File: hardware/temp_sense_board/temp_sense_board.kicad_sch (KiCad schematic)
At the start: 3 parts

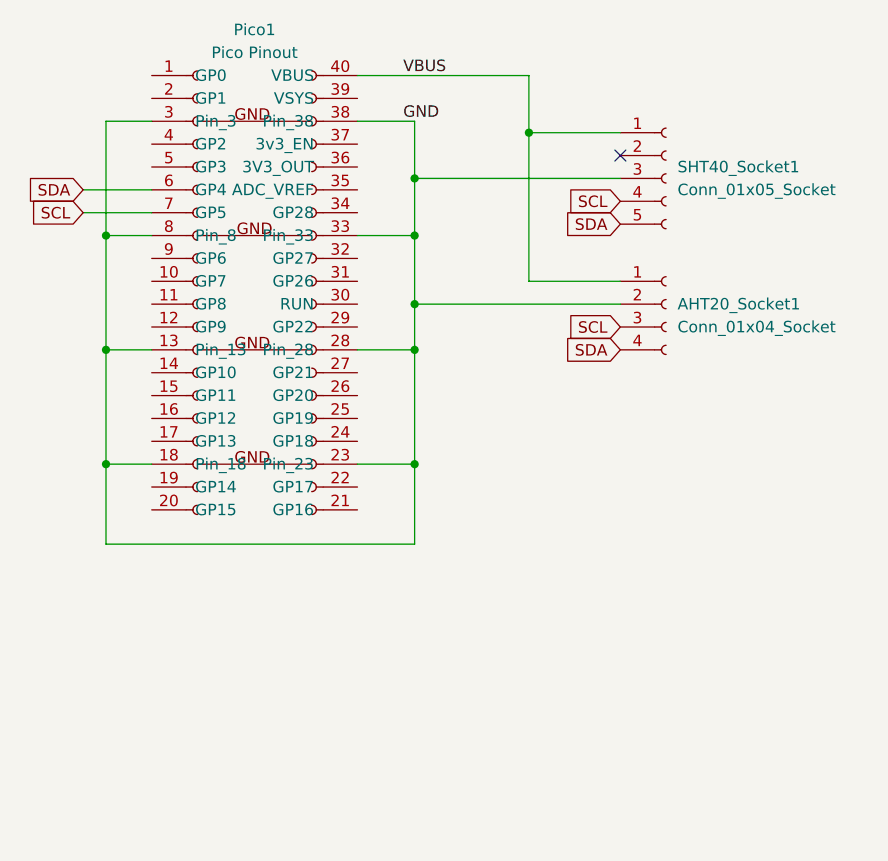
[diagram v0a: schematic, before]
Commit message: Updated PCB and Schematic
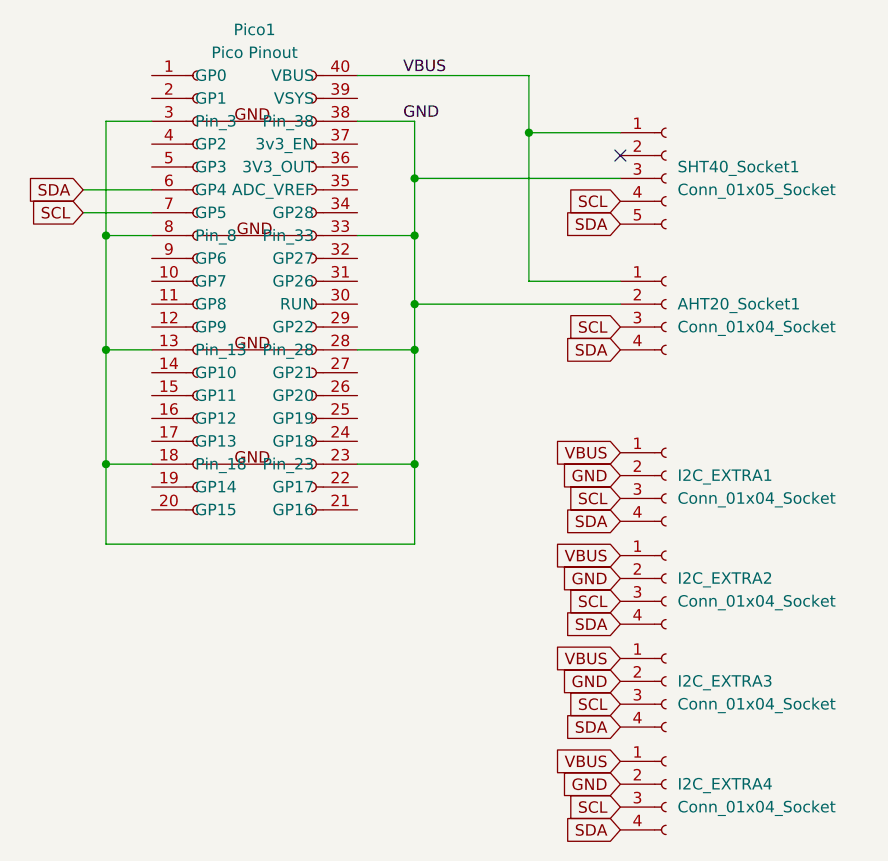
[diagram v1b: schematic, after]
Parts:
- added I2C_EXTRA1, I2C_EXTRA2, I2C_EXTRA3, I2C_EXTRA4: Conn_01x04_Socket, Connector_PinSocket_2.54mm:PinSocket_1x04_P2.54mm_Vertical, symbol Connector:Conn_01x04_Socket
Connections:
- net GND: now also I2C_EXTRA1.2 (Pin_2), I2C_EXTRA2.2 (Pin_2), I2C_EXTRA3.2 (Pin_2), I2C_EXTRA4.2 (Pin_2)
- net SCL: now also I2C_EXTRA1.3 (Pin_3), I2C_EXTRA2.3 (Pin_3), I2C_EXTRA3.3 (Pin_3), I2C_EXTRA4.3 (Pin_3)
- net SDA: now also I2C_EXTRA1.4 (Pin_4), I2C_EXTRA2.4 (Pin_4), I2C_EXTRA3.4 (Pin_4), I2C_EXTRA4.4 (Pin_4)
- net VBUS: now also I2C_EXTRA1.1 (Pin_1), I2C_EXTRA2.1 (Pin_1), I2C_EXTRA3.1 (Pin_1), I2C_EXTRA4.1 (Pin_1)
